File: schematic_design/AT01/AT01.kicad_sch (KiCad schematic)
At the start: 25 parts, among them J1 JST Connector, M2 Motor_DC (Pump), M3 Motor_DC (Solenoid), P1 USB_C_Plug_USB2.0, Q1 DMG2301L, SW1 SW_Push, U1 MPRLS0025PA00001A, U2 FT232RL, U3 DRV8833PW

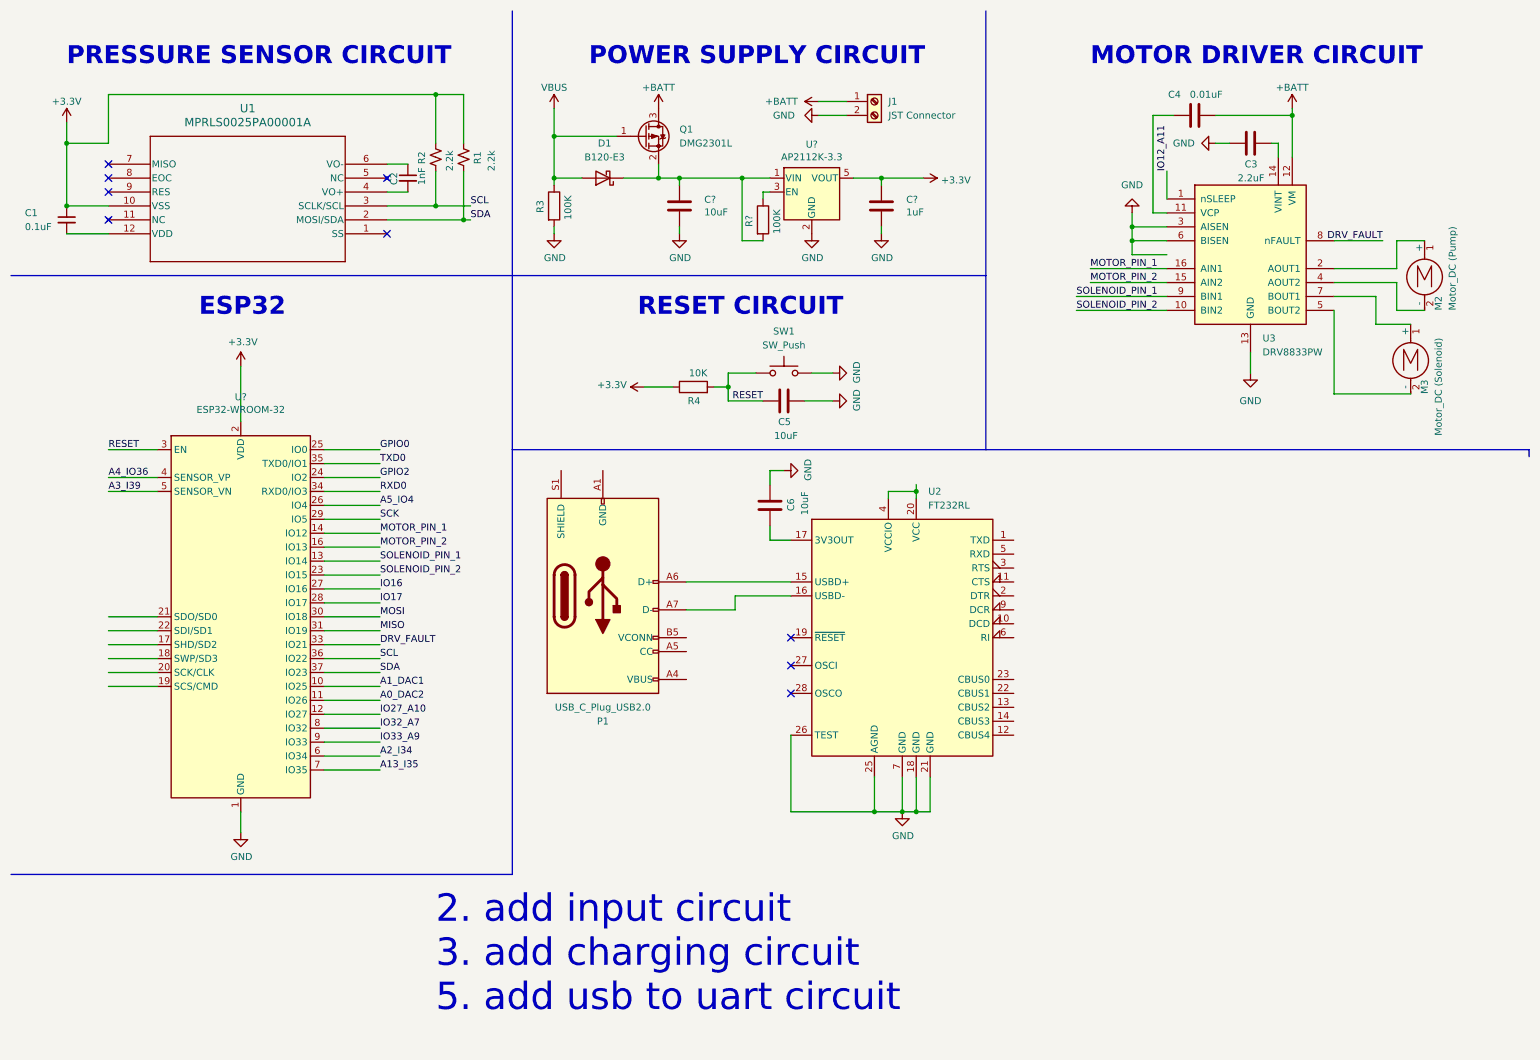
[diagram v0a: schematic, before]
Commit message: completed initial schematic development
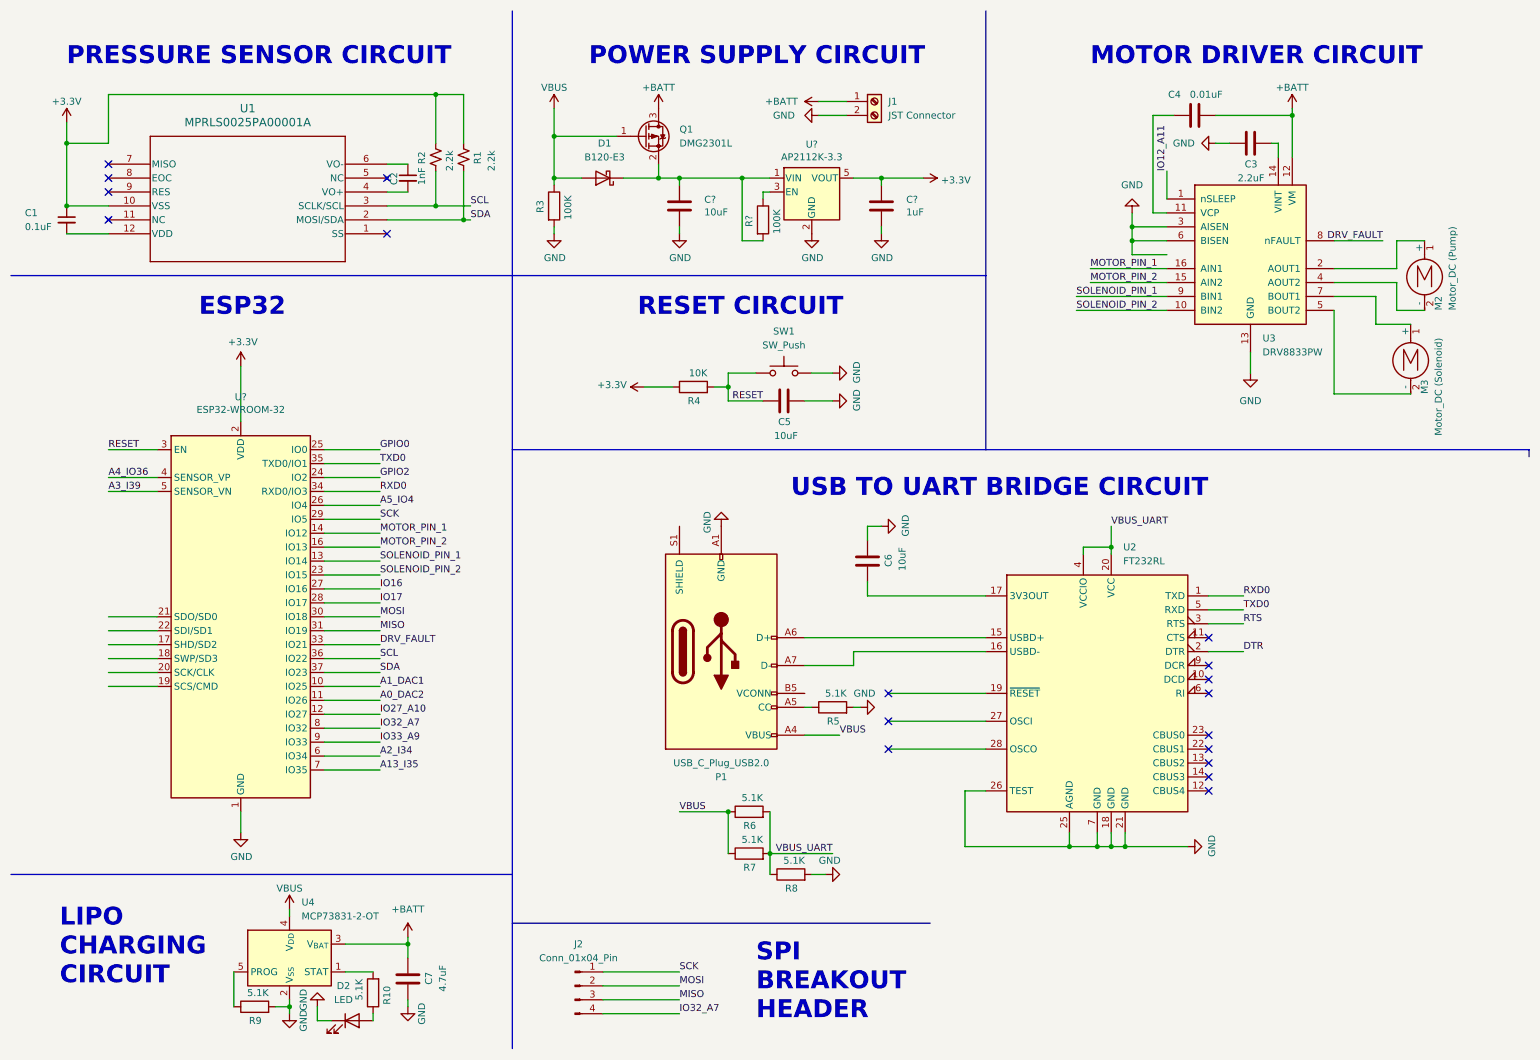
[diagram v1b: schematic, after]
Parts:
- added C7: 4.7uF, symbol Device:C
- added D2: LED, symbol Device:LED
- added J2: Conn_01x04_Pin, symbol Connector:Conn_01x04_Pin
- added R10, R5, R6, R7, R8, R9: 5.1K, symbol Device:R
- added U4: MCP73831-2-OT, Package_TO_SOT_SMD:SOT-23-5, symbol Battery_Management:MCP73831-2-OT
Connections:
- net +BATT: now also C7.2, U4.3 (V_{BAT})
- net GND: now also P1.A1 (GND), P1.A12 (GND), P1.B1 (GND), P1.B12 (GND), C7.1, D2.1 (K), R5.2, R8.2, R9.2, U4.2 (V_{SS})
- net IO32_A7: now also J2.4 (Pin_4)
- net MISO: now also J2.3 (Pin_3)
- net MOSI: now also J2.2 (Pin_2)
- net RXD0: now also U2.1 (TXD)
- net SCK: now also J2.1 (Pin_1)
- net TXD0: now also U2.5 (RXD)
- net VBUS: now also P1.A4 (VBUS), P1.A9 (VBUS), P1.B4 (VBUS), P1.B9 (VBUS), R6.1, R7.1, U4.4 (V_{DD})
- net DTR: now reaches U2.2 (DTR)
- net VBUS_UART: now reaches U2.20 (VCC), U2.4 (VCCIO)
- net VBUS_UART: now also R6.2, R7.2, R8.1
- net RTS: now reaches U2.3 (RTS)
- net at P1.A5 (CC): now also R5.1
- new net: D2.2 (A), R10.1
- new net: R10.2, U4.1 (STAT)
- new net: R9.1, U4.5 (PROG)
- no-connect marks 9 -> 18
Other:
- note added: "LIPO CHARGING CIRCUIT"
- note added: "SPI BREAKOUT HEADER"
- note added: "USB TO UART BRIDGE CIRCUIT"
- note removed: "2. add input circuit 3. add charging circuit 5. add usb to uart circuit"
- title: (none) -> AT01 - Initial Revision
- moved on the sheet: C6, P1, U2
